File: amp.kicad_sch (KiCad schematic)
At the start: 22 parts, among them J4 PinHeader_1x2_P2.54mm_Drill1.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, J5 Phone_TRS_MiniJack_SJ-3523-SM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, U3 TAS2505IRGER, Y2 Oscillator_50MHz_ECS_1612MV

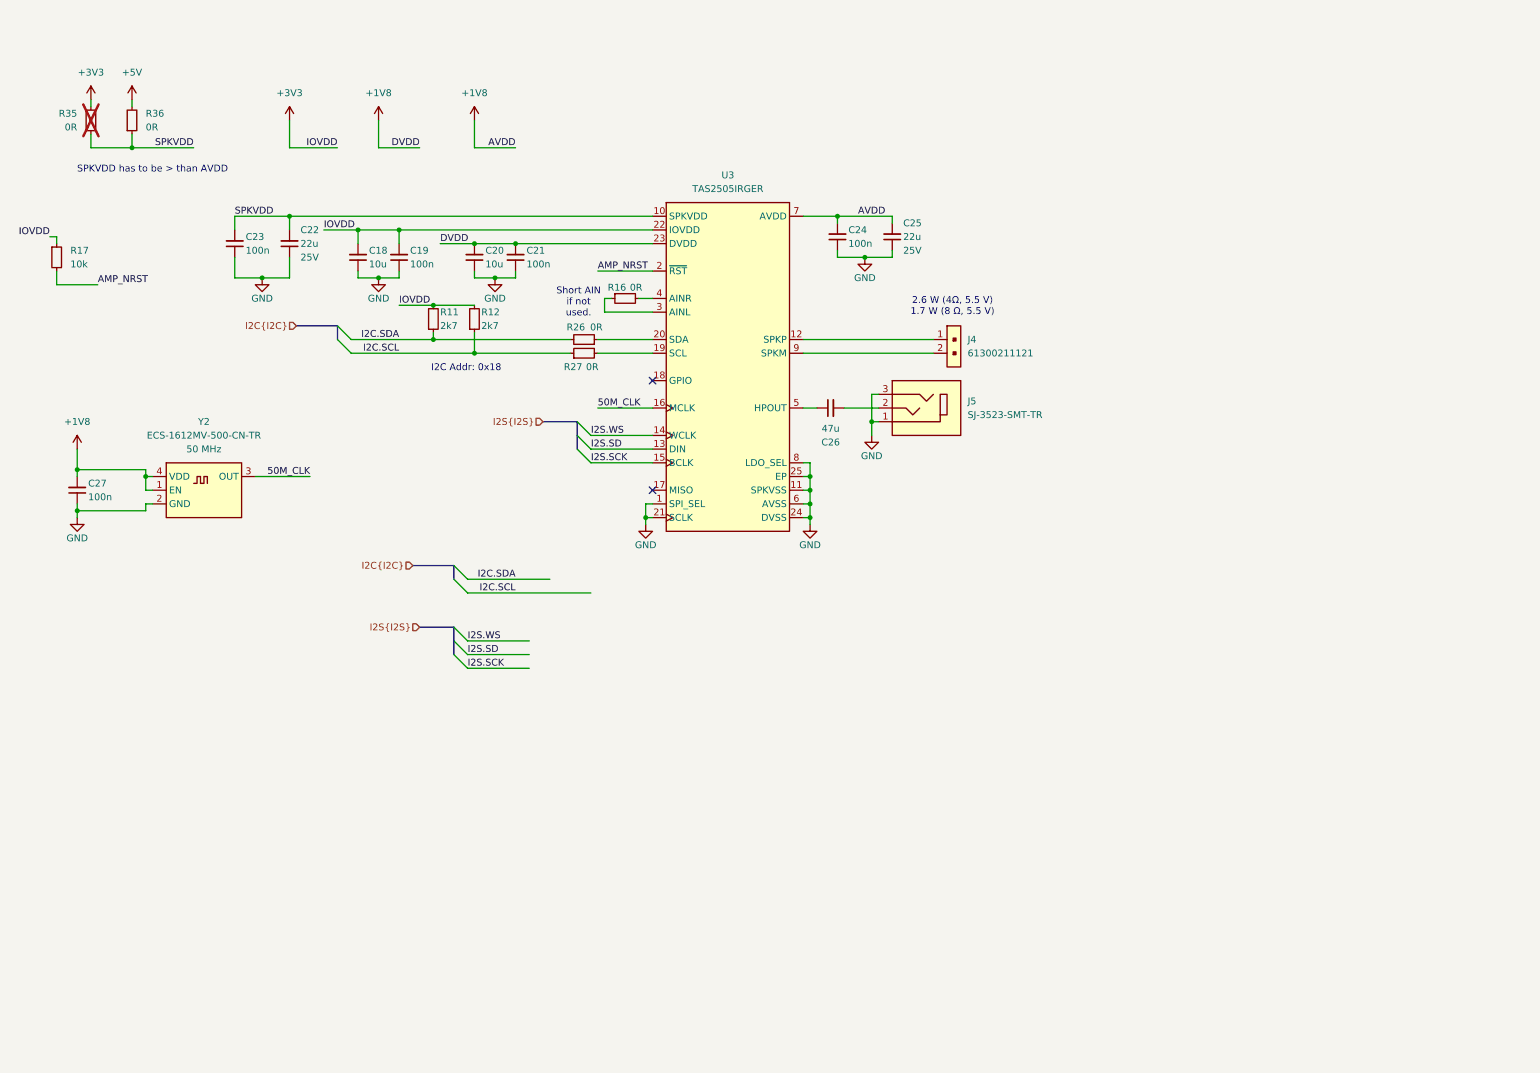
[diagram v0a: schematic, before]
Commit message: [#71555] Prepare sch for AMP
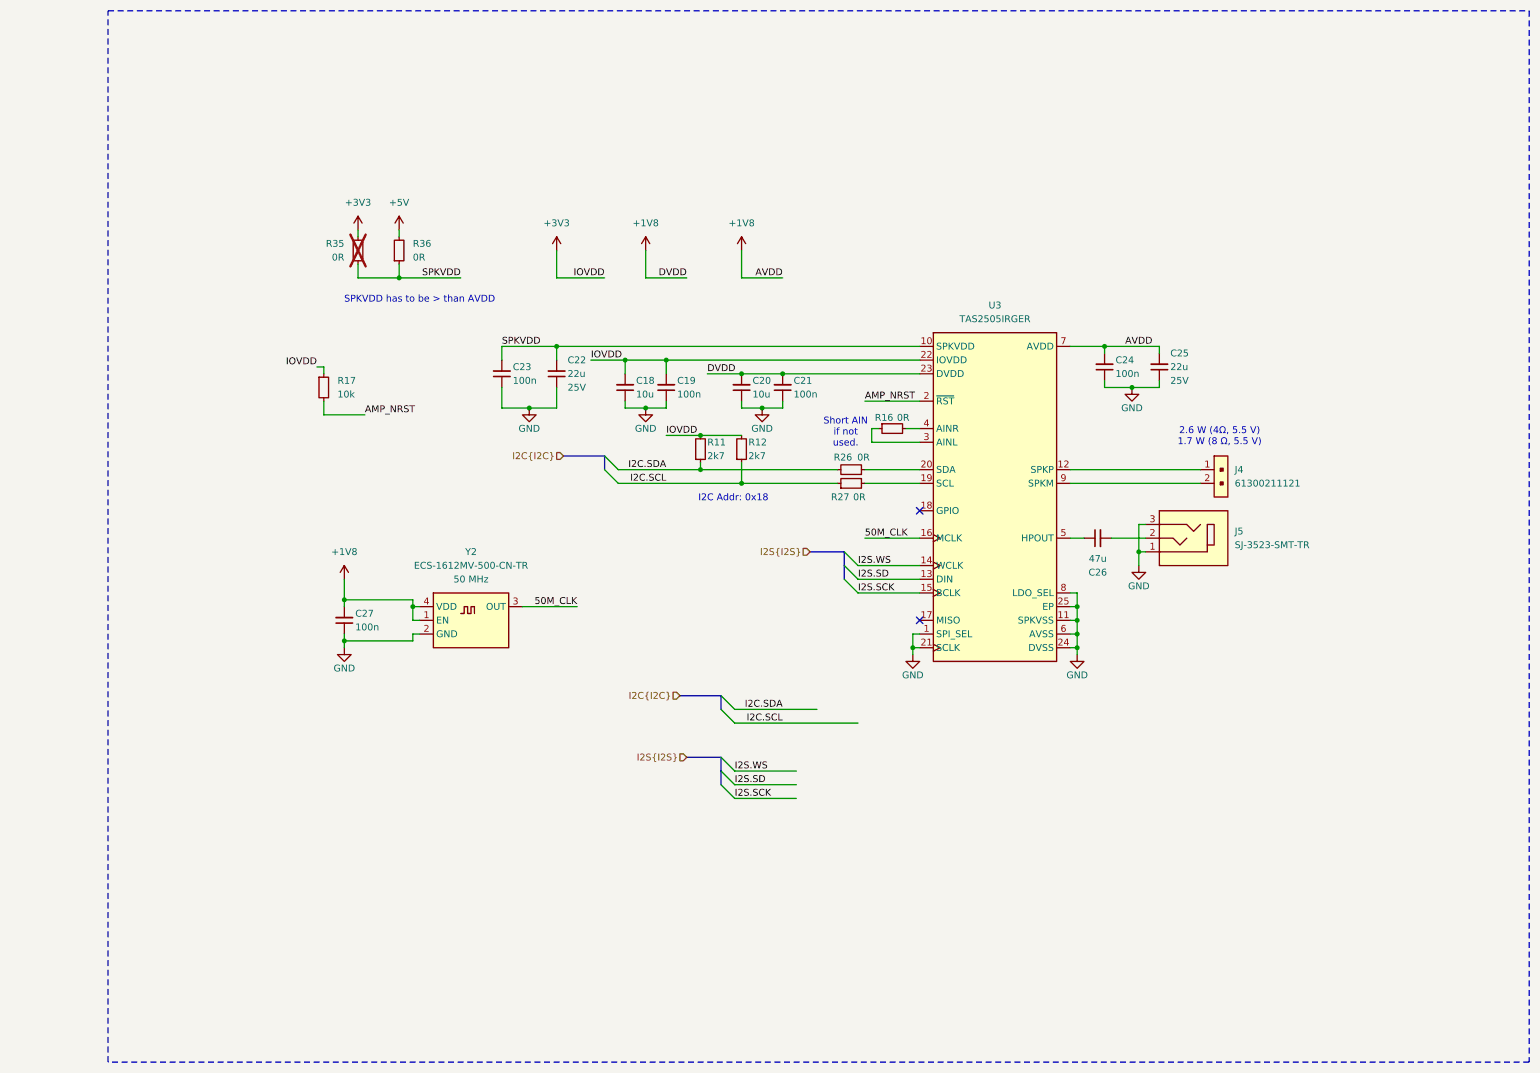
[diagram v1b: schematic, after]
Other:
- moved on the sheet: C18, C19, C20, C21, C22, C23, C24, C25, C26, C27, J4, J5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
